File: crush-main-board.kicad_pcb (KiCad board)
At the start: 4 copper layers, 38 parts, among them J1 4x4_Header, J10 3x3 Header, J11 3x3 Header, J12 3x2 Header, J13 3x4_Header, J14 3x4_Header, J15 2157601008, J2 4x4_Header, J3 6x2_Header, J4 3x1_Header, J5 3x2 Header, J6 3x2 Header, J7 3x4 Header, J8 3x4 Header, J9 3x3 Header, Q1 BSN20, Q2 BSN20, U1 Teensy4.1, U2 ISO7740DW, U3 ISO7740DW, U4 MCP3221A5T-I/OT, U5 ISO1640DBR

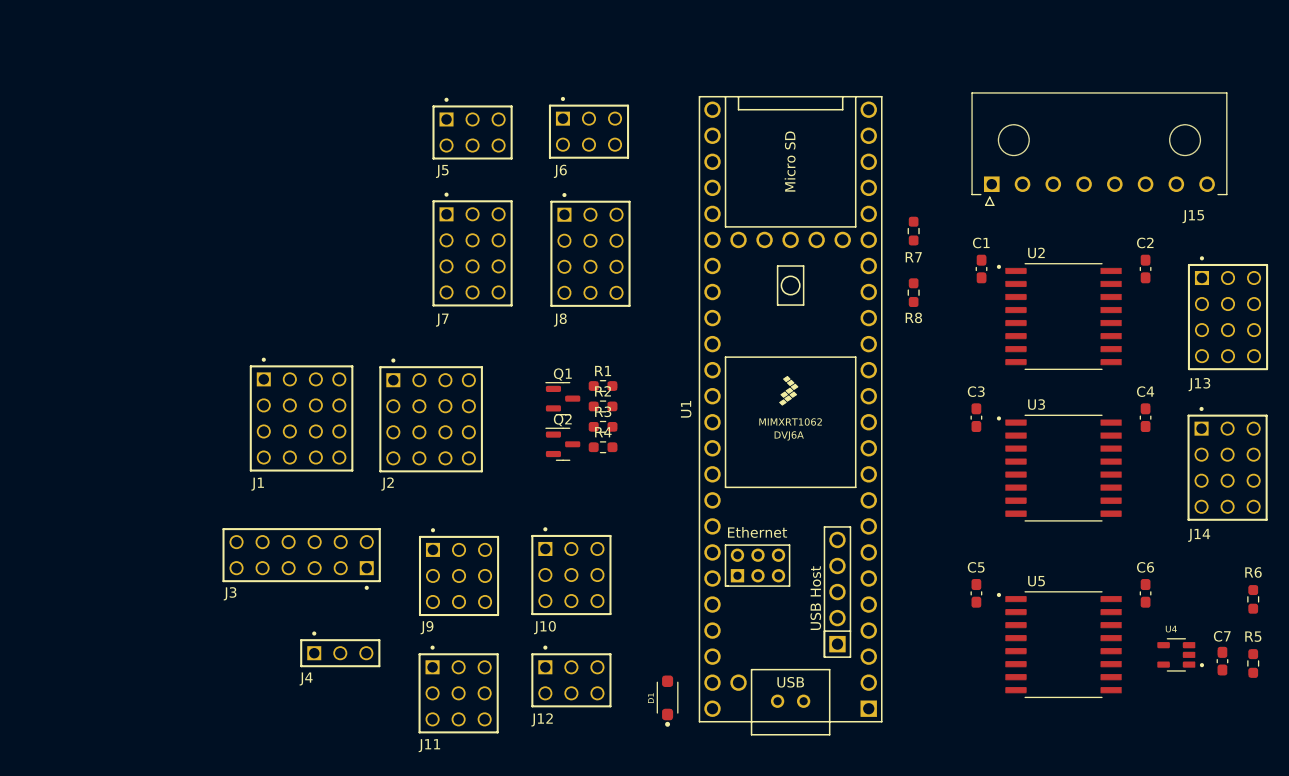
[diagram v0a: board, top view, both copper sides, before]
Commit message: arranged all components to be ready for routing
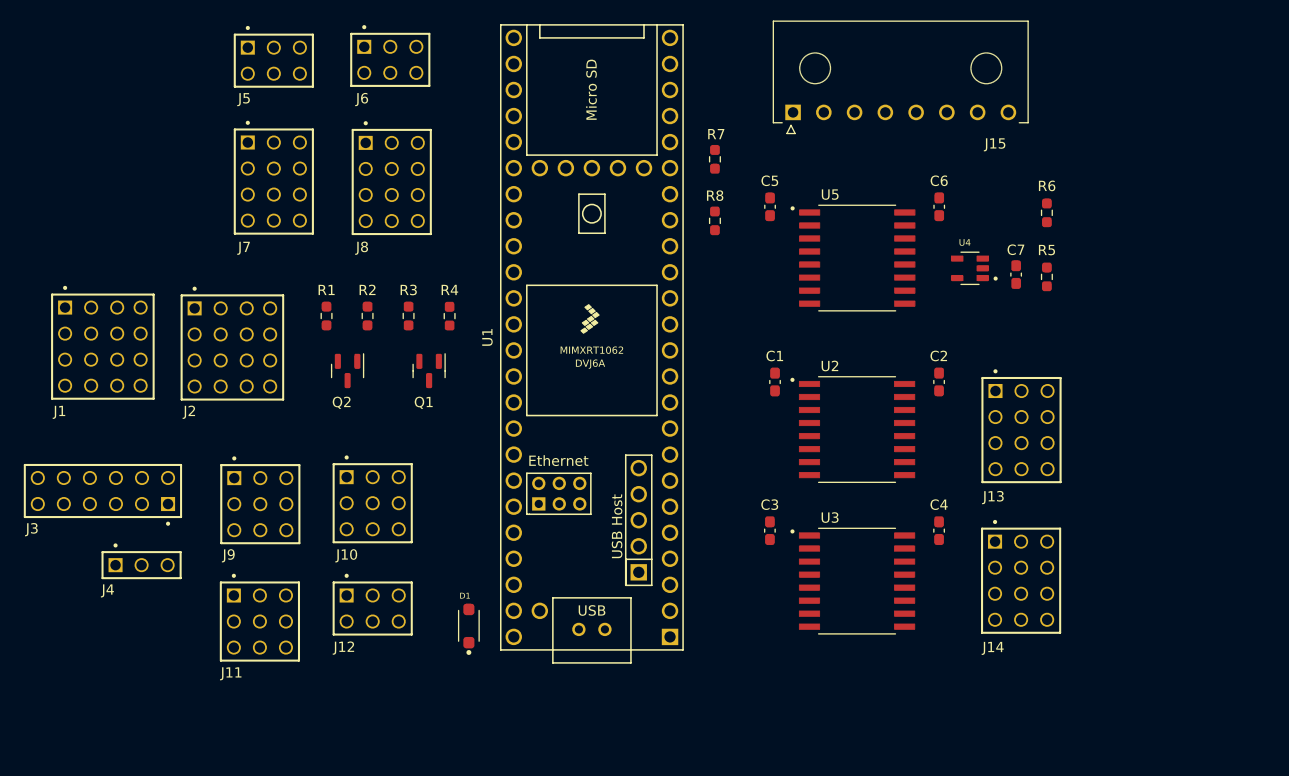
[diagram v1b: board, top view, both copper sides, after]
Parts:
- moved R5 42.7 mm to (184.4, 56.4)
- moved R6 42.7 mm to (184.4, 50.1)
- moved C5 42.7 mm to (157.4, 49.5)
- moved C6 42.7 mm to (173.9, 49.5)
- moved C7 42.7 mm to (181.4, 56.2)
- moved U4 42.7 mm to (176.9, 55.5)
- moved U5 42.7 mm to (165.9, 54.5)
- moved R1 27.8 mm to (114.1, 60.2), turned to -90 degrees
- moved R2 24.6 mm to (118.1, 60.2), turned to -90 degrees
- moved C1 23.0 mm to (157.9, 66.6)
- moved C2 23.0 mm to (173.9, 66.6)
- moved C3 23.0 mm to (157.4, 81.1)
- moved C4 23.0 mm to (173.9, 81.1)
- moved J14 23.0 mm to (181.9, 86.0)
- moved U2 23.0 mm to (165.9, 71.3)
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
